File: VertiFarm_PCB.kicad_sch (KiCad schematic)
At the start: 33 parts, among them J1 Peltier, J10 Raspberry Pi 5, J11 Peltier, J13 3V3 I2C, J15 3V3 I2C, J17 3V3 I2C, J18 5V I2C, J19 3V3 I2C, J20 Switch_2, J21 Camera, J22 DS12B20, J23 DS12B20, J24 DS12B20, J25 DS12B20, J26 DHT22, J27 DHT22, J33 left, J34 right, J5 Switch_1, J9 5V I2C

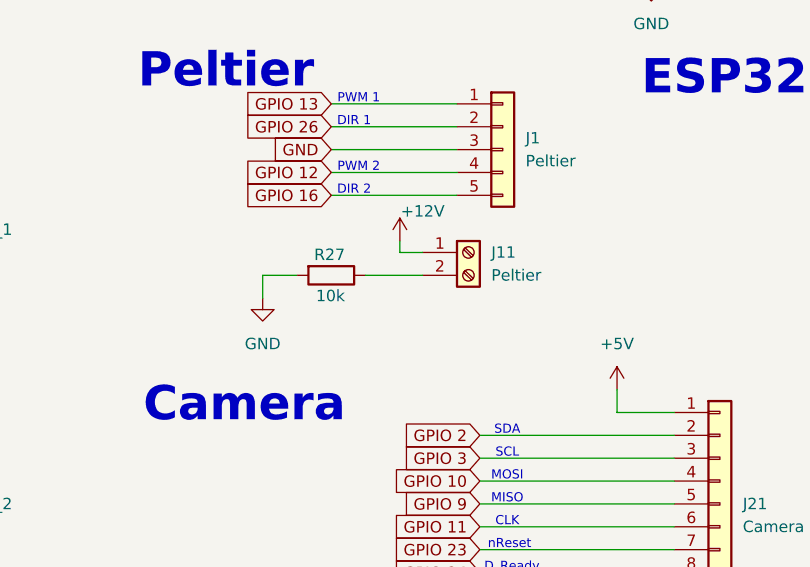
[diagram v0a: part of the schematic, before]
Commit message: Version 2.0
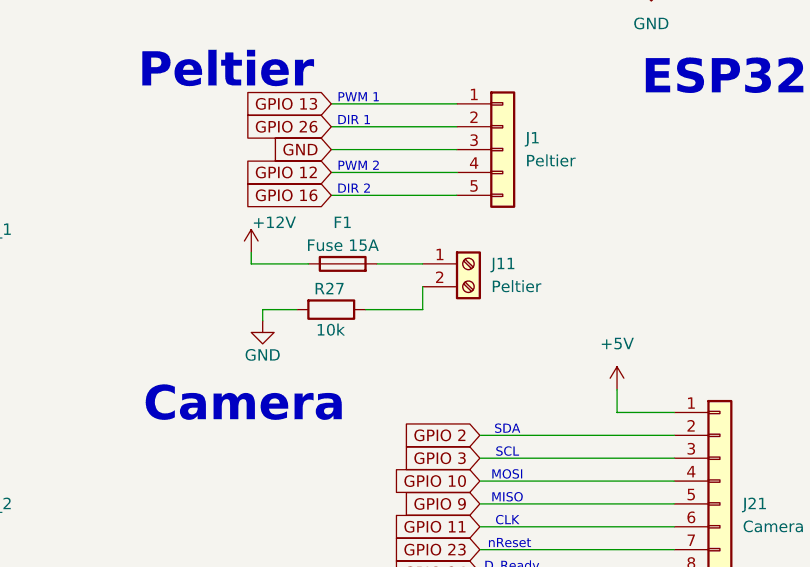
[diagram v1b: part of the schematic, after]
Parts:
- added F1: Fuse 15A, Fuse_Blade:Fuse_Blade_ATO_directSolder_32V_15A, symbol Device:Fuse
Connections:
- net +12V: now also F1.1; no longer J11.1 (Pin_1)
- new net: F1.2, J11.1 (Pin_1)
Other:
- moved on the sheet: J11, R27
